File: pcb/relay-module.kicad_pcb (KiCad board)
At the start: 4 copper layers, 50 x 50 mm, 92 parts, among them J1 AVR-UPDI-6, J2 QWICC, J3 Power In, J4 Power Out, K1 PR24-5V-900-1A, P1 MountingHole_Pad, P2 MountingHole_Pad, P3 MountingHole_Pad, P4 MountingHole_Pad, Q1 MMBT3904, U1 ATtiny1616-MNR, U3 LTV-356T

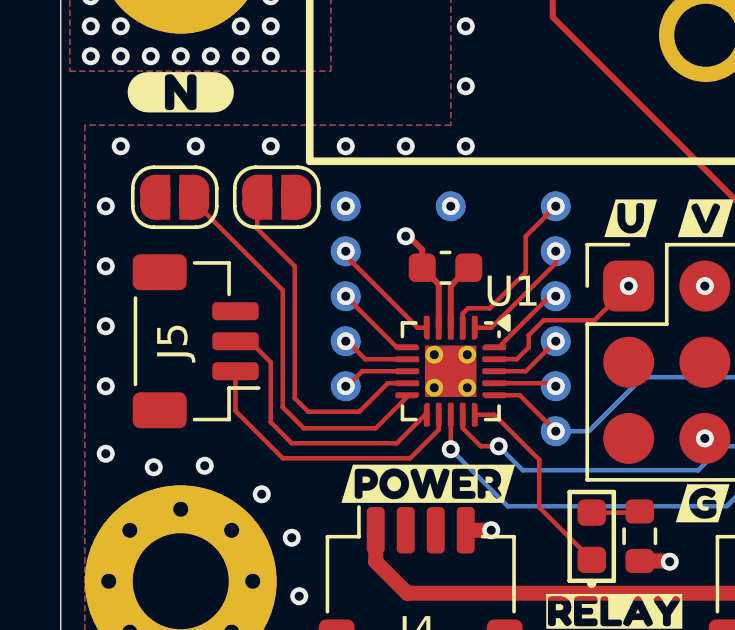
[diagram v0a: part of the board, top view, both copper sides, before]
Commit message: schematic and PCB clean up
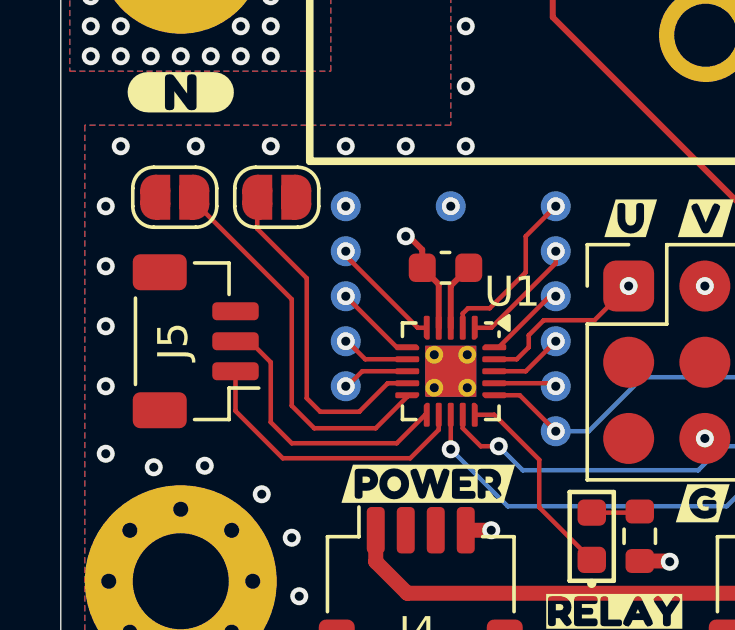
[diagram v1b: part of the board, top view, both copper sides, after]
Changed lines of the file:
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@@
 				(font
 					(size 0.001 0.001)
+					(thickness 0.15)
 				)
 			)
@@
 				(font
 					(size 0.001 0.001)
+					(thickness 0.15)
 				)
 			)
@@
 				(font
 					(size 0.001 0.001)
+					(thickness 0.15)
 				)
 				(justify mirror)
@@
 				(font
 					(size 0.001 0.001)
+					(thickness 0.15)
 				)
 				(justify mirror)
@@
 				(font
 					(size 0.001 0.001)
+					(thickness 0.15)
 				)
 				(justify mirror)
@@
 				(font
 					(size 0.001 0.001)
+					(thickness 0.15)
 				)
 				(justify mirror)
@@
 				(font
 					(size 0.001 0.001)
+					(thickness 0.15)
 				)
 				(justify mirror)
@@
 				(font
 					(size 0.001 0.001)
+					(thickness 0.15)
 				)
 				(justify mirror)
@@
 				(font
 					(size 0.001 0.001)
+					(thickness 0.15)
 				)
 				(justify mirror)
@@
 				(font
 					(size 0.001 0.001)
+					(thickness 0.15)
 				)
 				(justify mirror)
@@
 				(font
 					(size 0.001 0.001)
+					(thickness 0.15)
 				)
 				(justify mirror)
@@
 				(font
 					(size 0.001 0.001)
+					(thickness 0.15)
 				)
 				(justify mirror)
@@
 				(font
 					(size 0.001 0.001)
+					(thickness 0.15)
 				)
 				(justify mirror)
@@
 				(font
 					(size 0.001 0.001)
+					(thickness 0.15)
 				)
 				(justify mirror)
@@
 				(font
 					(size 0.001 0.001)
+					(thickness 0.15)
 				)
 				(justify mirror)
@@
 				(font
 					(size 0.001 0.001)
+					(thickness 0.15)
 				)
 				(justify mirror)
@@
 				(font
 					(size 0.001 0.001)
+					(thickness 0.15)
 				)
 				(justify mirror)
@@
 				(font
 					(size 0.001 0.001)
+					(thickness 0.15)
 				)
 				(justify mirror)
@@
 				(font
 					(size 0.001 0.001)
+					(thickness 0.15)
 				)
 				(justify mirror)
@@
 				(font
 					(size 0.001 0.001)
+					(thickness 0.15)
 				)
 				(justify mirror)
@@
 				(font
 					(size 0.001 0.001)
+					(thickness 0.15)
 				)
 				(justify mirror)
@@
 				(font
 					(size 0.001 0.001)
+					(thickness 0.15)
 				)
 				(justify mirror)
@@
 				(font
 					(size 0.001 0.001)
+					(thickness 0.15)
 				)
 				(justify mirror)
@@
 				(font
 					(size 0.001 0.001)
+					(thickness 0.15)
 				)
 				(justify mirror)
@@
 				(font
 					(size 0.001 0.001)
+					(thickness 0.15)
 				)
 				(justify mirror)
@@
 				(font
 					(size 0.001 0.001)
+					(thickness 0.15)
 				)
 				(justify mirror)
@@
 				(font
 					(size 0.001 0.001)
+					(thickness 0.15)
 				)
 				(justify mirror)
@@
 				(font
 					(size 0.001 0.001)
+					(thickness 0.15)
 				)
 				(justify mirror)
@@
 				(font
 					(size 0.001 0.001)
+					(thickness 0.15)
 				)
 				(justify mirror)
@@
 				(font
 					(size 0.001 0.001)
+					(thickness 0.15)
 				)
 				(justify mirror)
@@
 	)
 	(segment
-		(start 58.1 140.9)
-		(end 60.5 140.9)
+		(start 60.5 140.9)
+		(end 61.55 139.85)
 		(width 0.1524)
 		(layer "F.Cu")
@@
 	)
 	(segment
-		(start 57.4 140.2)
-		(end 58.1 140.9)
+		(start 57.7 140.15)
+		(end 58.45 140.9)
 		(width 0.1524)
 		(layer "F.Cu")
@@
 	)
 	(segment
-		(start 57.4 136.3)
-		(end 57.4 140.2)
+		(start 61.55 139.85)
+		(end 61.55 139.8)
 		(width 0.1524)
 		(layer "F.Cu")
@@
 	)
 	(segment
-		(start 54.45 133.35)
-		(end 57.4 136.3)
+		(start 54.45 133.2)
+		(end 54.45 133.35)
 		(width 0.1524)
 		(layer "F.Cu")
@@
 	)
 	(segment
-		(start 61.55 139.85)
-		(end 61.55 139.8)
+		(start 54.45 133.35)
+		(end 57.7 136.6)
 		(width 0.1524)
 		(layer "F.Cu")
@@
 	)
 	(segment
-		(start 60.5 140.9)
-		(end 61.55 139.85)
+		(start 57.7 136.6)
+		(end 57.7 140.15)
 		(width 0.1524)
 		(layer "F.Cu")
@@
 	)
 	(segment
-		(start 54.45 133.2)
-		(end 54.45 133.35)
+		(start 58.45 140.9)
+		(end 60.5 140.9)
 		(width 0.1524)
 		(layer "F.Cu")
@@
 	)
 	(segment
-		(start 58.25 140.35)
-		(end 59.95 140.35)
+		(start 59.95 140.35)
+		(end 60.9 139.4)
 		(width 0.1524)
 		(layer "F.Cu")
@@
 	)
 	(segment
-		(start 57.8 139.9)
-		(end 58.25 140.35)
+		(start 58.2 139.9)
+		(end 58.65 140.35)
 		(width 0.1524)
 		(layer "F.Cu")
@@
 	)
 	(segment
-		(start 56.55 134.25)
-		(end 57.8 135.5)
+		(start 60.9 139.4)
+		(end 61.55 139.4)
 		(width 0.1524)
 		(layer "F.Cu")
@@
 	)
 	(segment
-		(start 59.95 140.35)
-		(end 60.9 139.4)
+		(start 58.65 140.35)
+		(end 59.95 140.35)
 		(width 0.1524)
 		(layer "F.Cu")
@@
 	)
 	(segment
-		(start 57.8 135.5)
-		(end 57.8 139.9)
+		(start 56.55 134.25)
+		(end 58.2 135.9)
 		(width 0.1524)
 		(layer "F.Cu")
@@
 	)
 	(segment
-		(start 60.9 139.4)
-		(end 61.55 139.4)
+		(start 58.2 135.9)
+		(end 58.2 139.9)
 		(width 0.1524)
 		(layer "F.Cu")
